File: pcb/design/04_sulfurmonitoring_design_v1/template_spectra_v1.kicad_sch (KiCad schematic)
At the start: 3 parts, among them U1 Heltec_WSL_V3

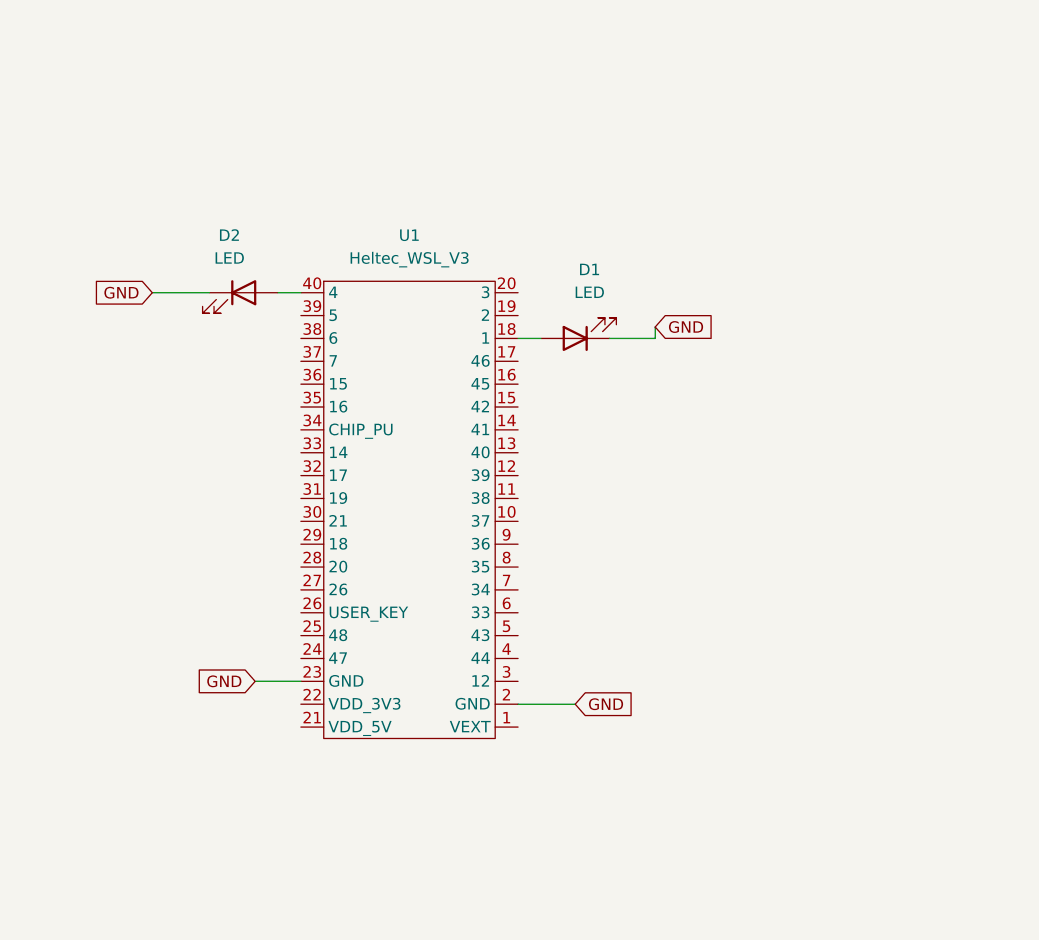
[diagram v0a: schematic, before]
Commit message: design
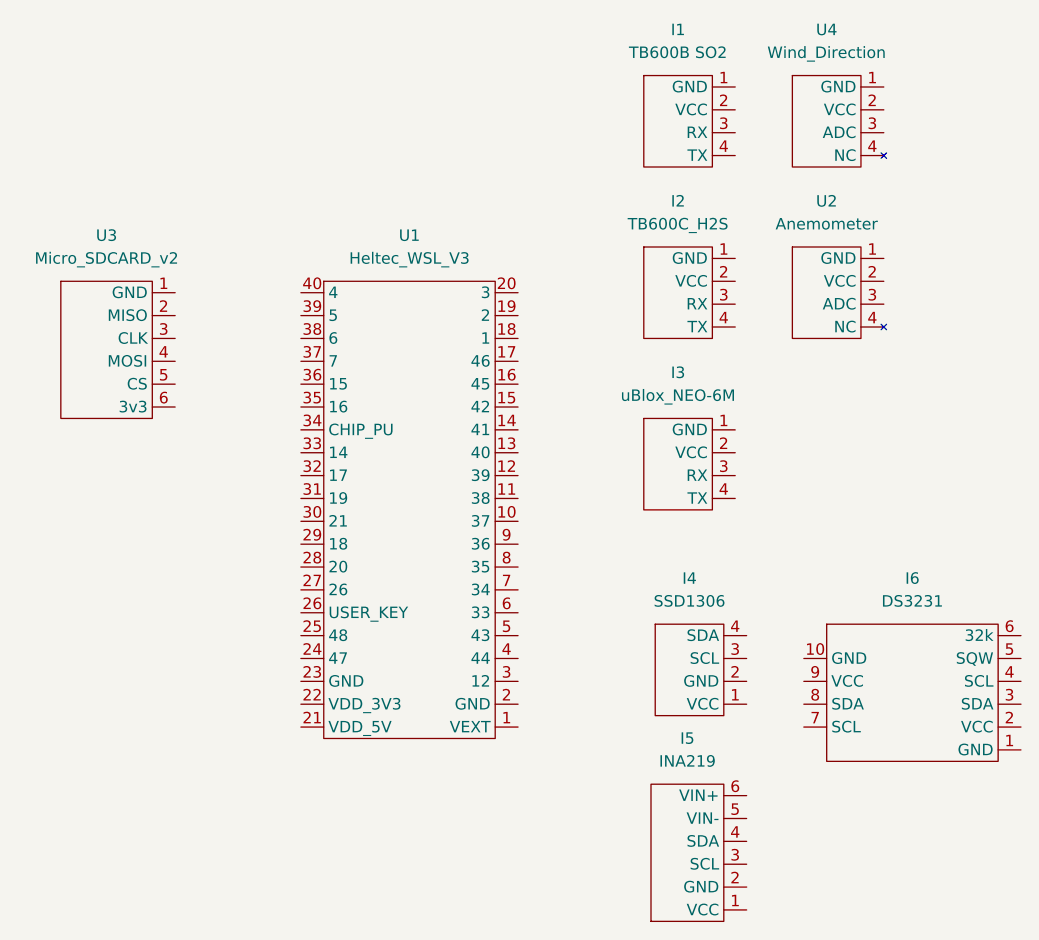
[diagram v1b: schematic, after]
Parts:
- removed D1, D2: LED, LED_THT:LED_D5.0mm, symbol Device:LED
- added I1: TB600B SO2, Custom Board:TB600B_SO2, symbol Custom Board:TB600B
- added I2: TB600C_H2S, Custom Board:TB600C_H2S, symbol Custom Board:TB600C
- added I3: uBlox_NEO-6M, Custom Board:uBlox_NEO-6M, symbol Custom Board:GPS
- added I4: SSD1306​, Custom Board:SSD1306_onBoard, symbol Custom Board:SSD1306​
- added I5: INA219, Custom Board:INA219, symbol Custom Board:INA219
- added I6: DS3231​, Custom Board:DS3231, symbol Custom Board:RTC_DS3231​
- added U2: Anemometer, Custom Board:STASRG_Anemometer, symbol Custom Board:Anemometer
- added U3: Micro_SDCARD_v2, Custom Board:Micro_SDCARD_v2, symbol Custom Board:SPI SD Card_v2
- added U4: Wind_Direction, Custom Board:STASRG_Wind_Dir, symbol Custom Board:Wind Direction
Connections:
- net GND: no longer names the net of U1.2 (GND)
- net GND: no longer U1.23 (GND)
